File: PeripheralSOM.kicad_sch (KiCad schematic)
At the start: 6 parts, among them J4 52465-2470

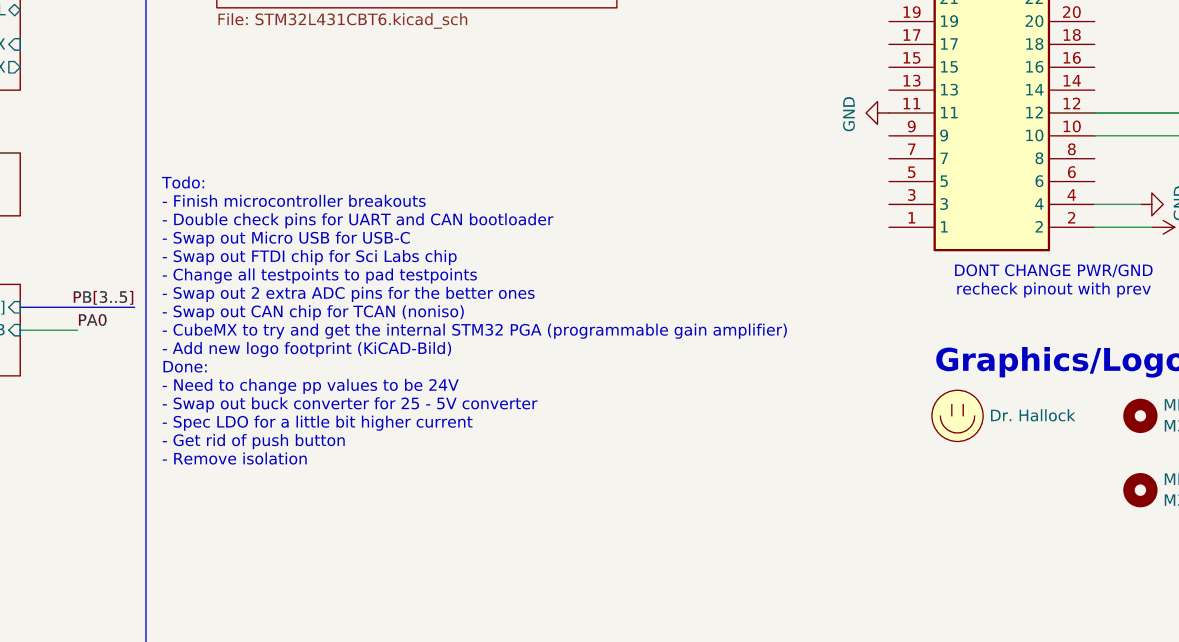
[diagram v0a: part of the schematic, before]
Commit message: add 5v power mux
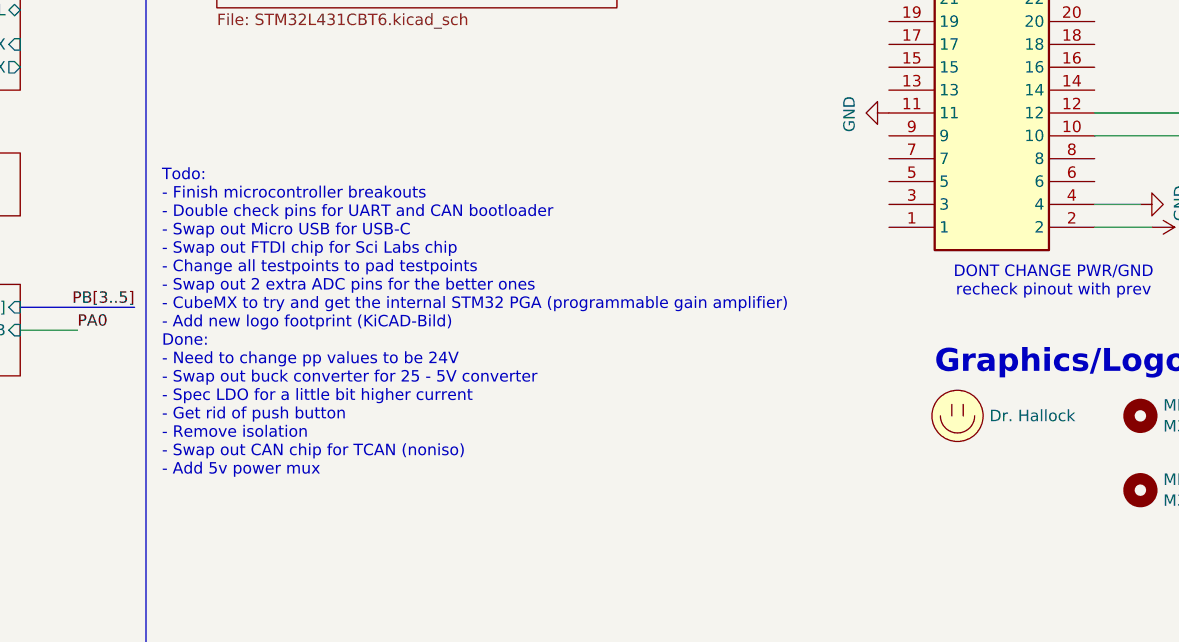
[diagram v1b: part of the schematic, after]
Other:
- note added: "Todo: - Finish microcontroller breakouts - Double check pins for UART and CAN bootloader - Swap out Micro USB for USB-C - Swap out FTDI chip for Sci Labs chip - Change all testpoints to pad testpoints - Swap out 2 extra ADC pins for the better ones - CubeMX to try and get the internal STM32 PGA (programmable gain amplifier) - Add new logo footprint (KiCAD-Bild) Done: - Need to change pp values to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"
- note removed: "Todo: - Finish microcontroller breakouts - Double check pins for UART and CAN bootloader - Swap out Micro USB for USB-C - Swap out FTDI chip for Sci Labs chip - Change all testpoints to pad testpoints - Swap out 2 extra ADC pins for the better ones - Swap out CAN chip for TCAN (noniso) - CubeMX to try and get the internal STM32 PGA (programmable gain amplifier) - Add new logo footprint (KiCAD-Bil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"
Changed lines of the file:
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@@
 		)
 	)
-	(text "Todo:\n- Finish microcontroller breakouts\n- Double check pins for UART and CAN bootloader\n- Swap out Micro USB for USB-C\n- Swap out FTDI chip for Sci Labs chip\n- Change all testpoints to pad testpoints\n- Swap out 2 extra ADC pins for the better ones\n- Swap out CAN chip for TCAN (noniso)\n- CubeMX to try and get the internal STM32 PGA (programmable gain amplifier)\n- Add new logo footprint (KiCAD-Bild)\nDone:\n- Need to change pp values to be 24V\n- Swap out buck converter for 25 - 5V converter\n- Spec LDO for a little bit higher current\n- Get rid of push button\n- Remove isolation\n"
+	(text "Todo:\n- Finish microcontroller breakouts\n- Double check pins for UART and CAN bootloader\n- Swap out Micro USB for USB-C\n- Swap out FTDI chip for Sci Labs chip\n- Change all testpoints to pad testpoints\n- Swap out 2 extra ADC pins for the better ones\n- CubeMX to try and get the internal STM32 PGA (programmable gain amplifier)\n- Add new logo footprint (KiCAD-Bild)\nDone:\n- Need to change pp values to be 24V\n- Swap out buck converter for 25 - 5V converter\n- Spec LDO for a little bit higher current\n- Get rid of push button\n- Remove isolation\n- Swap out CAN chip for TCAN (noniso)\n- Add 5v power mux"
 		(exclude_from_sim no)
 		(at 69.088 79.248 0)
